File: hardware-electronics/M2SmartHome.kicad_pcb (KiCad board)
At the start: 4 copper layers, 22 x 76 mm, 207 parts, among them J1 M.2-Key-M-edge-connector, J2 Micro_SD_Card_Det_Hirose_DM3AT, J3 CONMHF1-SMD-T, J4 CONMHF1-SMD-T, U1 RTL8188FTV-VC-CG, U10 24AA04T-I_OT, U2 EMMC16G-MW28-01E10, U3 PI7C9X440SLBFDE, U4 24AA04T-I_OT, U5 CP2102N-A02-GQFN20, U6 24AA04T-I_OT, U7 EFR32MG21B020F1024IM32-B, U8 USB2244-AEZG-06, U9 USB2244-AEZG-06, Y1 ABM8-12.000MHZ-B2-T, Y2 ECS-240-10-47-CKM-TR, Y3 ECS-240-10-47-CKM-TR, Y5 ABM8-40.000MHZ-B2-T

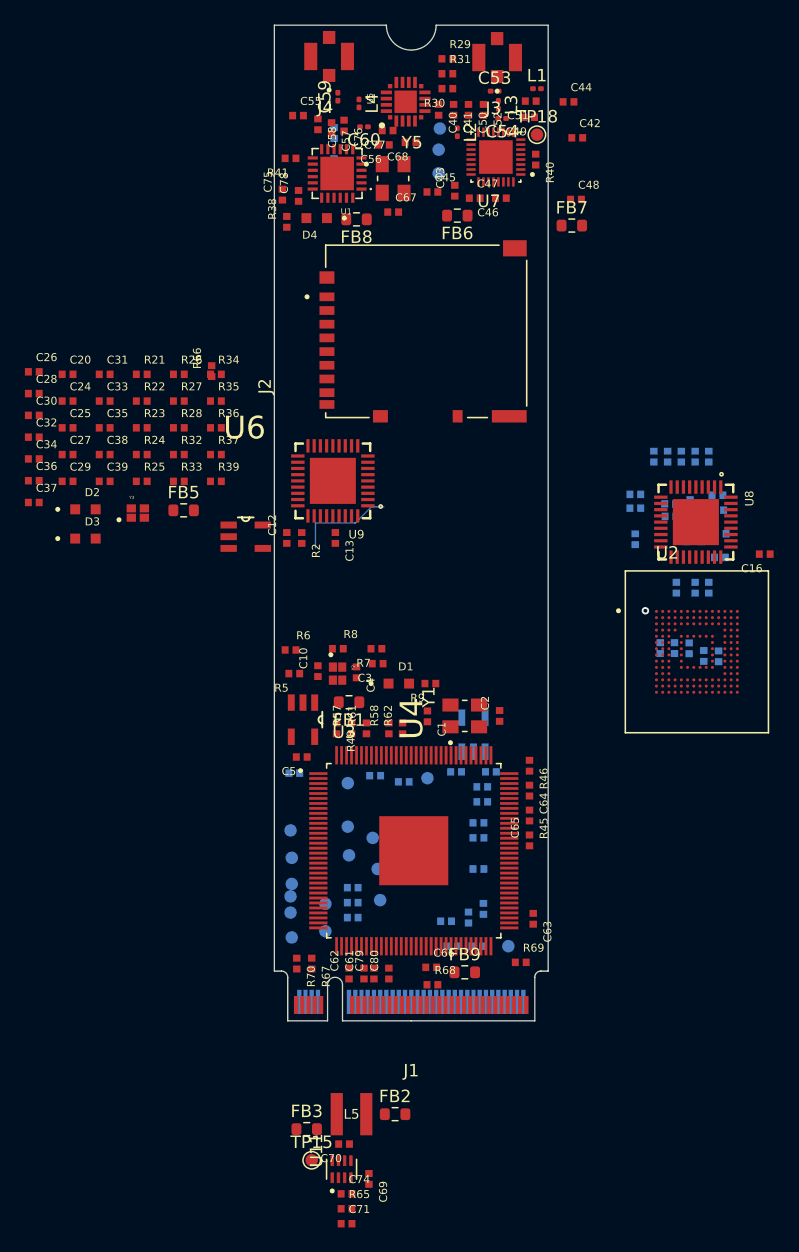
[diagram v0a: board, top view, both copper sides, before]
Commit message: [#13] WIP Placement eMMC
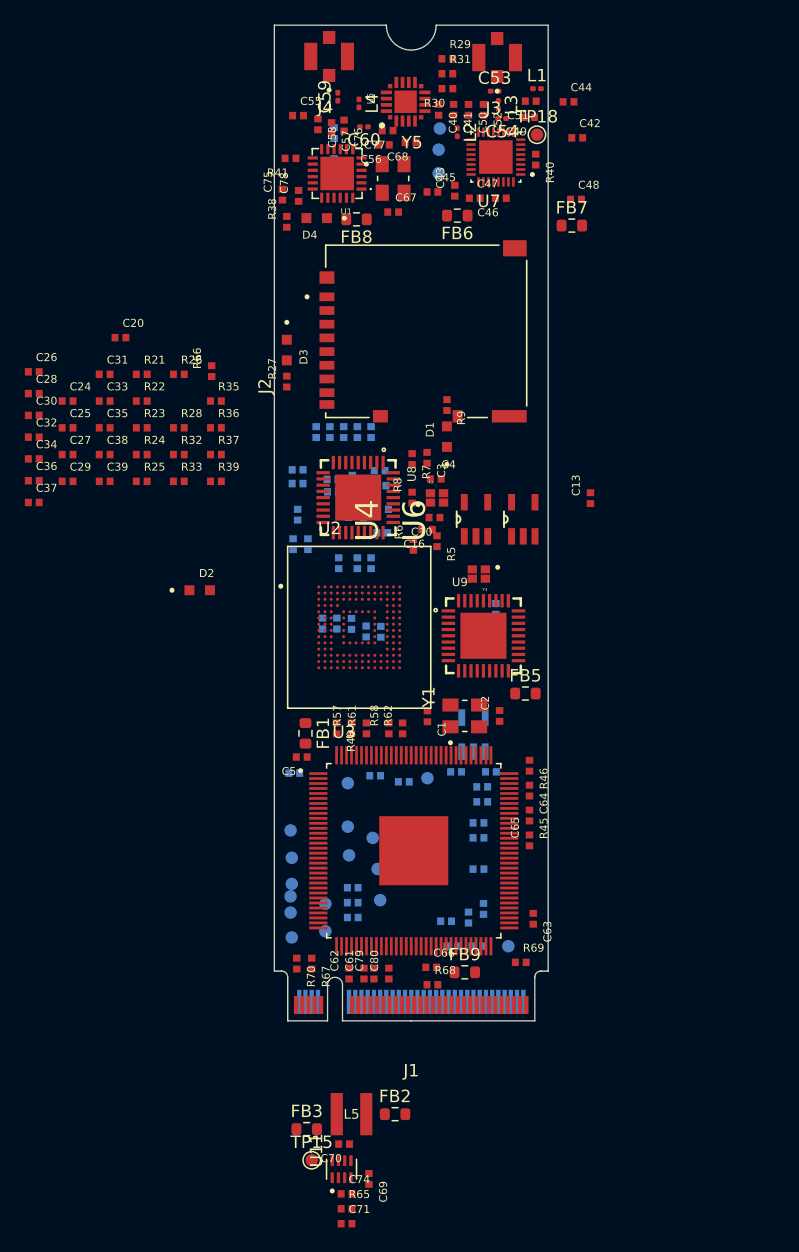
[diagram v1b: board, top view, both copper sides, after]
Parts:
- C12, R2, R34: moved to B.Cu
- moved FB5 31.2 mm to (101.2, 139.7)
- moved R34 29.3 mm to (98.8, 132.9), turned to 90 degrees
- moved Y3 27.8 mm to (97.4, 130.1), turned to 180 degrees
- moved C15 27.2 mm to (86.0, 134.1)
- moved C16 27.2 mm to (93.3, 126.5)
- moved C8 27.2 mm to (87.3, 122.6)
- moved C9 27.2 mm to (89.5, 123.0)
- moved R12 27.2 mm to (88.8, 118.7)
- moved R13 27.2 mm to (88.8, 129.2)
- moved R18 27.2 mm to (86.6, 118.7)
- moved U2 27.2 mm to (87.8, 134.4)
- moved U8 27.2 mm to (87.7, 124.0)
- moved R11 27.2 mm to (87.7, 118.7)
- moved R17 27.2 mm to (85.5, 118.7)
- moved R19 27.2 mm to (84.4, 118.7)
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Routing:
- net Net-(U2-DAT4): track 8.04 -> 0.00 mm, vias 1 -> 0
